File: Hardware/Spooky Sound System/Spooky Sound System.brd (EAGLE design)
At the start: 101.6 x 36.5 mm, 37 parts, among them P1 100K, P2 100K, P3 100K, U1 TDA7387, U2 AZ4558C, U3 AZ4558C

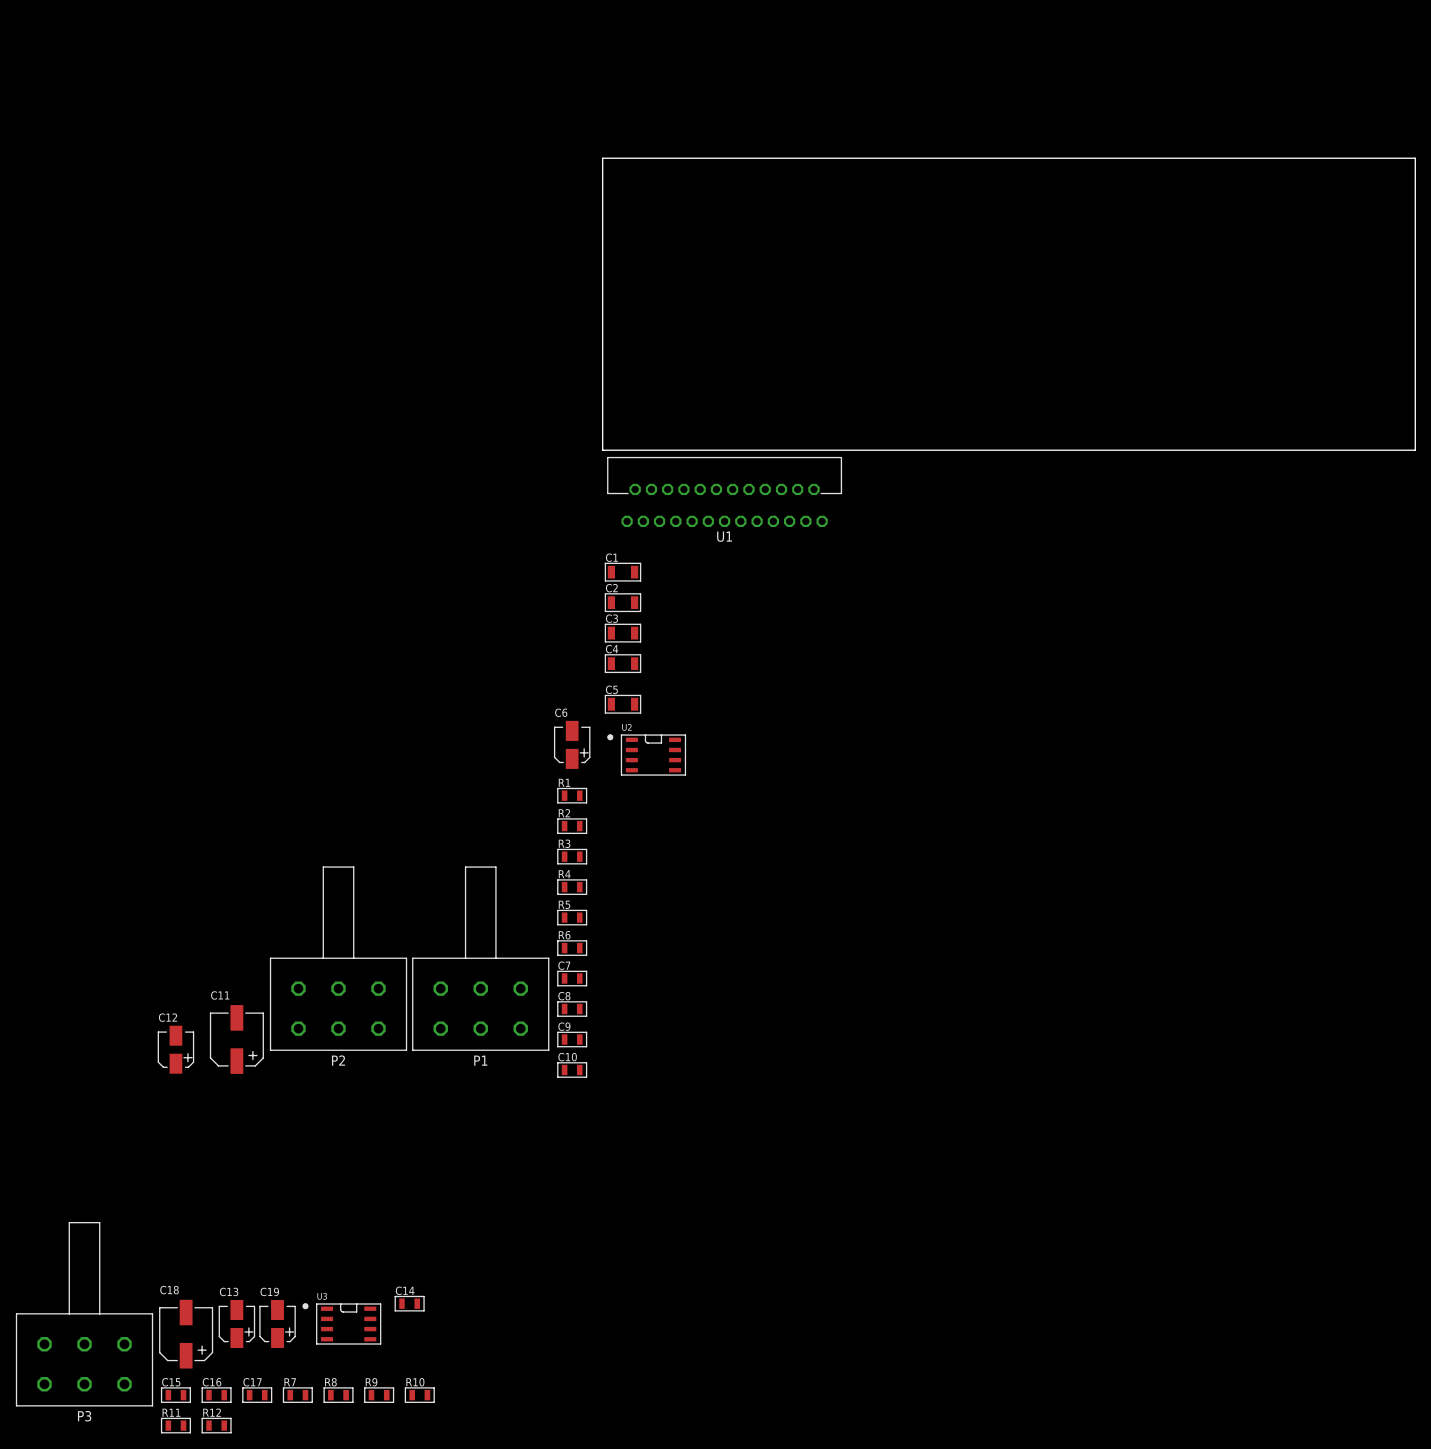
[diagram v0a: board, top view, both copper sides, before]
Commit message: Schematic done. Start Routing.
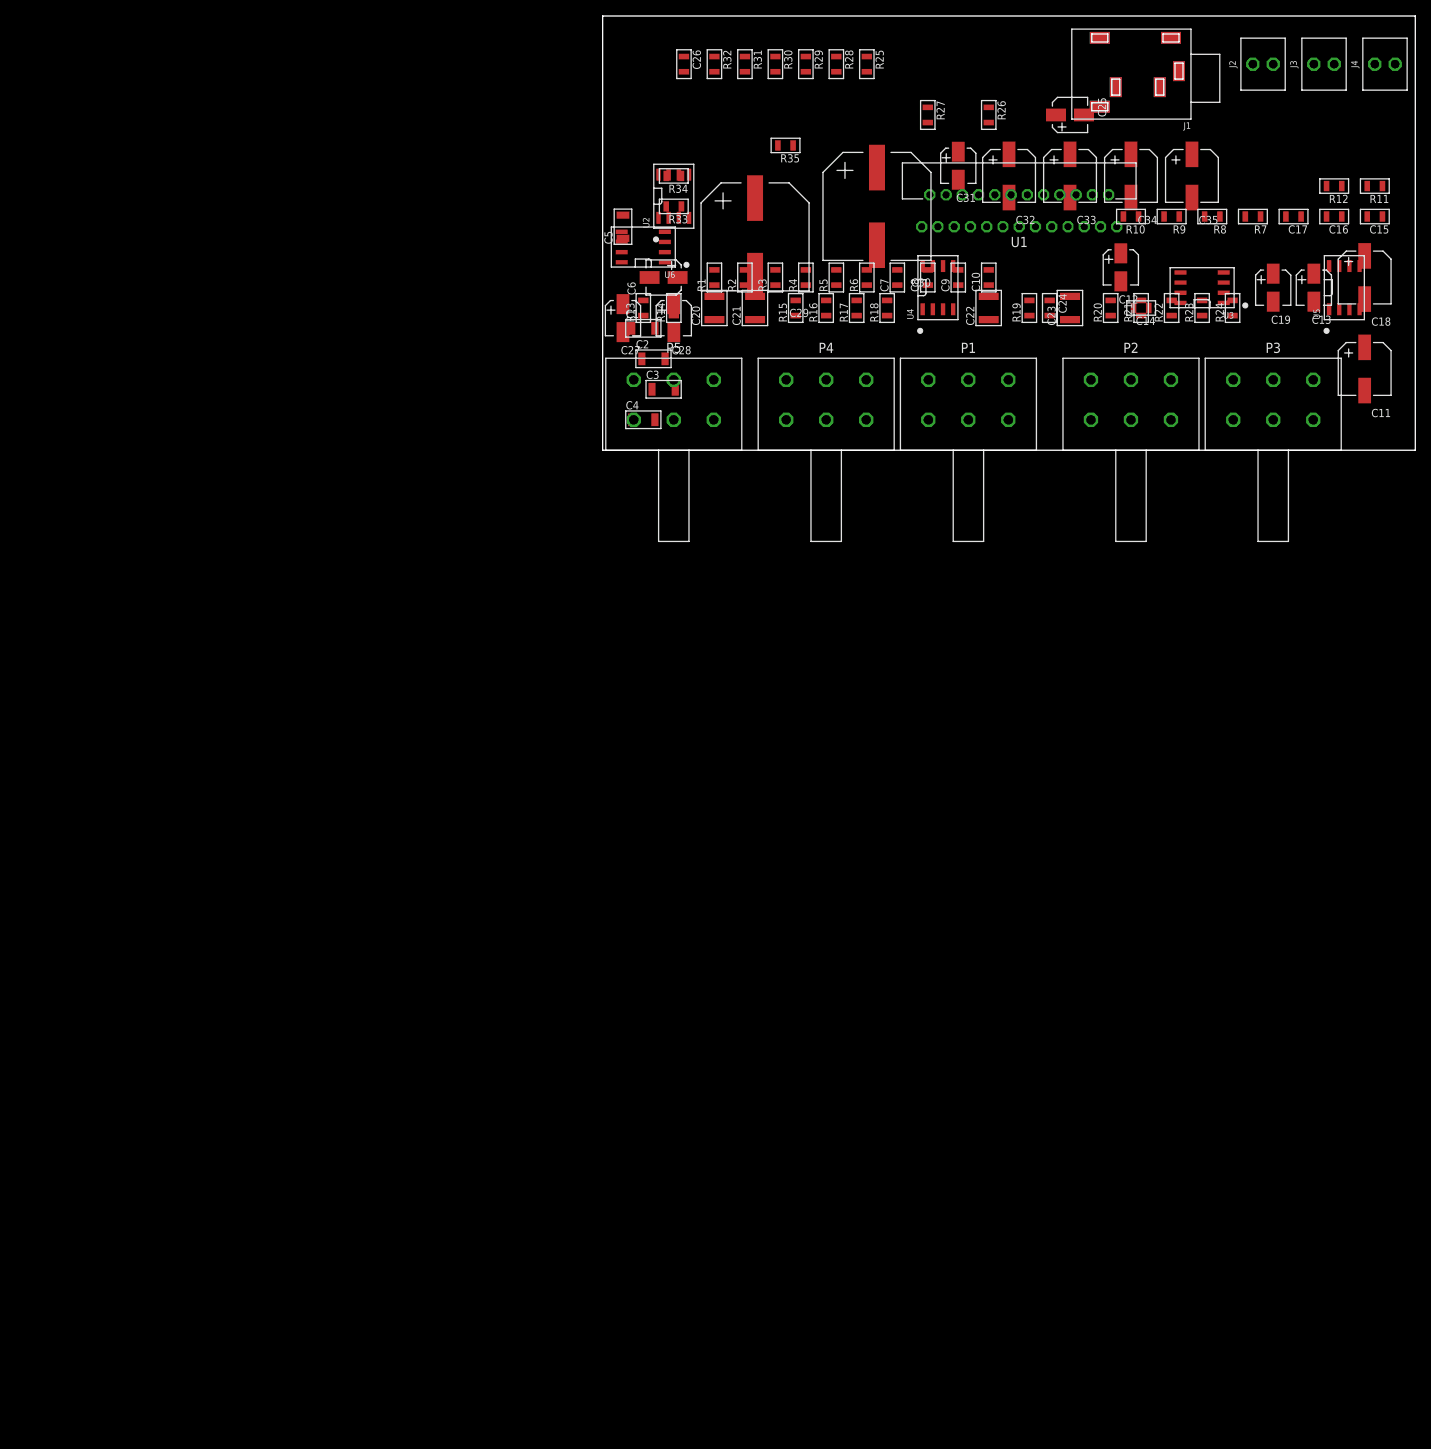
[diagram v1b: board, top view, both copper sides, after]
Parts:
- added C20, C21, C22, C23: 0.01uF, MF_Passives:C1210
- added C24: 22nF, MF_Passives:C0805
- added C25, C27, C28, C31: 10uF, MF_Passives:CP4MM
- added C26: 0.1uF, MF_Passives:C0805
- added C29, C30: 1000uF, MF_Passives:CP12.5MM
- added C32: 47uF, MF_Passives:CP6.3MM
- added C33, C34, C35: 100uF, MF_Passives:CP6.3MM
- added J1: SJ1-3533NS, PP_Connectors:SJ1-3533NS
- added J2, J3, J4: 1546215-2, PP_Connectors:1546215-2
- added P4, P5: 100K, PP_Passives:DUAL_TAPER_POTENTIOMETER
- added R13, R14, R19, R20: 1M, MF_Passives:R0805
- added R15, R16, R17, R18, R21, R22, R23, R24, R27, R30, R31, R32: 0, MF_Passives:R0805
- added R25, R26, R28, R29: 10K, MF_Passives:R0805
- added R33, R34: 220K, MF_Passives:R0805
- added R35: 1K, MF_Passives:R0805
- added U4, U5, U6: AZ4558C, PP_AnalogIC:AZ4558C_SOIC-8
- moved R11 215.6 mm to (96.5, 33.0), turned to 180 degrees
- moved C15 210.1 mm to (96.5, 29.2), turned to 180 degrees
- moved R12 208.6 mm to (91.4, 33.0), turned to 180 degrees
- moved C16 203.0 mm to (91.4, 29.2), turned to 180 degrees
- moved C18 197.9 mm to (95.2, 21.6), turned to 180 degrees
- moved C17 196.2 mm to (86.4, 29.2), turned to 180 degrees
- moved R7 189.6 mm to (81.3, 29.2), turned to 180 degrees
- moved C13 186.8 mm to (88.9, 20.3), turned to 180 degrees
- moved P3 183.7 mm to (83.8, 0.00), turned to 180 degrees
- moved R8 183.4 mm to (76.2, 29.2), turned to 180 degrees
- moved C19 179.6 mm to (83.8, 20.3), turned to 180 degrees
- moved R9 177.5 mm to (71.1, 29.2), turned to 180 degrees
- moved R10 172.1 mm to (66.0, 29.2), turned to 180 degrees
- moved U3 167.8 mm to (74.9, 20.3), turned to 180 degrees
- moved C11 164.0 mm to (95.2, 10.2), turned to 180 degrees
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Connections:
- new net AUD_IN_L: C20.P$1, C22.P$1, J1.2_A, J1.2_B
- new net AUD_IN_R: C21.P$1, C23.P$1, J1.3_A, J1.3_B
- new net L+: J2.P$1, U1.P$9
- new net L-: J2.P$2, U1.P$7
- new net N$23: C27.P$2, R21.P$2, U4.1
- new net N$24: P5.3A, R21.P$1
- new net N$25: P3.3B, R16.P$1
- new net N$26: P3.1B, R17.P$2
- new net N$27: C28.P$2, R23.P$2, U4.7
- new net N$28: P5.3B, R23.P$1
- new net N$29: C26.P$1, R25.P$2, R26.P$2, R28.P$1, U5.2
- new net N$30: C26.P$2, P4.3A, R28.P$2, U5.1
- new net N$31: R29.P$1, U5.3
- new net N$32: P4.2A, R31.P$2
- new net N$33: R30.P$2, R32.P$1, U5.6
- new net N$34: C25.P$1, R30.P$1, U5.7
- new net N$35: P5.2A, U4.2
- new net N$36: P5.1A, R22.P$2
- new net N$37: P5.1B, R24.P$2
- new net N$38: P5.2B, U4.6
- new net N$39: P3.2B, U3.2
- new net N$40: P3.3A, R18.P$2
- new net N$41: P3.2A, U2.2
- new net N$42: P3.1A, R15.P$1
- new net N$43: C24.P$1, R31.P$1, U5.5
- new net N$44: C25.P$2, R27.P$1
- new net N$45: C27.P$1, R26.P$1
- new net N$46: C28.P$1, R25.P$1
- new net N$47: C33.P$2, C34.P$1, R33.P$2, R34.P$1, U6.3
- new net N$48: R35.P$1, U6.1
- new net N$49: C32.P$1, U1.P$10
- new net OUT_SUB: C3.P$1, R27.P$2
- new net R+: J3.P$1, U1.P$5
- new net R-: J3.P$2, U1.P$3
- new net SUB+: J4.P$1, U1.P$17
- new net SUB-: J4.P$2, U1.P$19
- new net SUB_L: C22.P$2, R19.P$1
- new net SUB_R: C23.P$2, R20.P$1, U4.5
- new net VGND: C11.P$2, C18.P$2, C24.P$2, R12.P$2, R13.P$2, R14.P$2, R17.P$1, R18.P$1, R19.P$2, R20.P$2, R22.P$1, R24.P$1, R29.P$2, R32.P$2, R35.P$2, R6.P$2, U6.2
- net GND: now also C29.P$2, C30.P$2, C31.P$2, C32.P$2, C34.P$2, C35.P$2, C4.P$1, C5.P$1, J1.1_A, J1.1_B, J1.S1, J1.S2, J1.S3, J1.S4, J1.S5, J1.S6, R34.P$2, U1.P$1, U1.P$13, U1.P$18, U1.P$2, U1.P$24, U1.P$8, U4.4, U5.4, U6.4; no longer C11.P$2, C18.P$2, P3.1A, P3.3B, R12.P$2, R6.P$2
- net IN_L: now also C20.P$2, R14.P$1
- net IN_R: now also C21.P$2, R13.P$1
- net N$1: now also R15.P$2; no longer U2.2
- net N$12: now also R16.P$2; no longer U3.2
- net OUT_L: now also C1.P$1; no longer P3.3A
- net OUT_R: now also C2.P$1; no longer P3.1B
- net VIN: now also C29.P$1, C30.P$1, C31.P$1, C33.P$1, C35.P$1, R33.P$1, U1.P$20, U1.P$22, U1.P$4, U1.P$6, U4.8, U5.8, U6.8
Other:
- board size 101.6 x 36.5 mm -> 101.6 x 54.3 mm
